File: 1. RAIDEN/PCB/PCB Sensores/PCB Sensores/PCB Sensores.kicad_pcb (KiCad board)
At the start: 2 copper layers, 61.4 x 100 mm, 19 parts, among them J2 LEDS_1, J3 LEDS_1, J4 LEDS_1, U1 BOB-09056

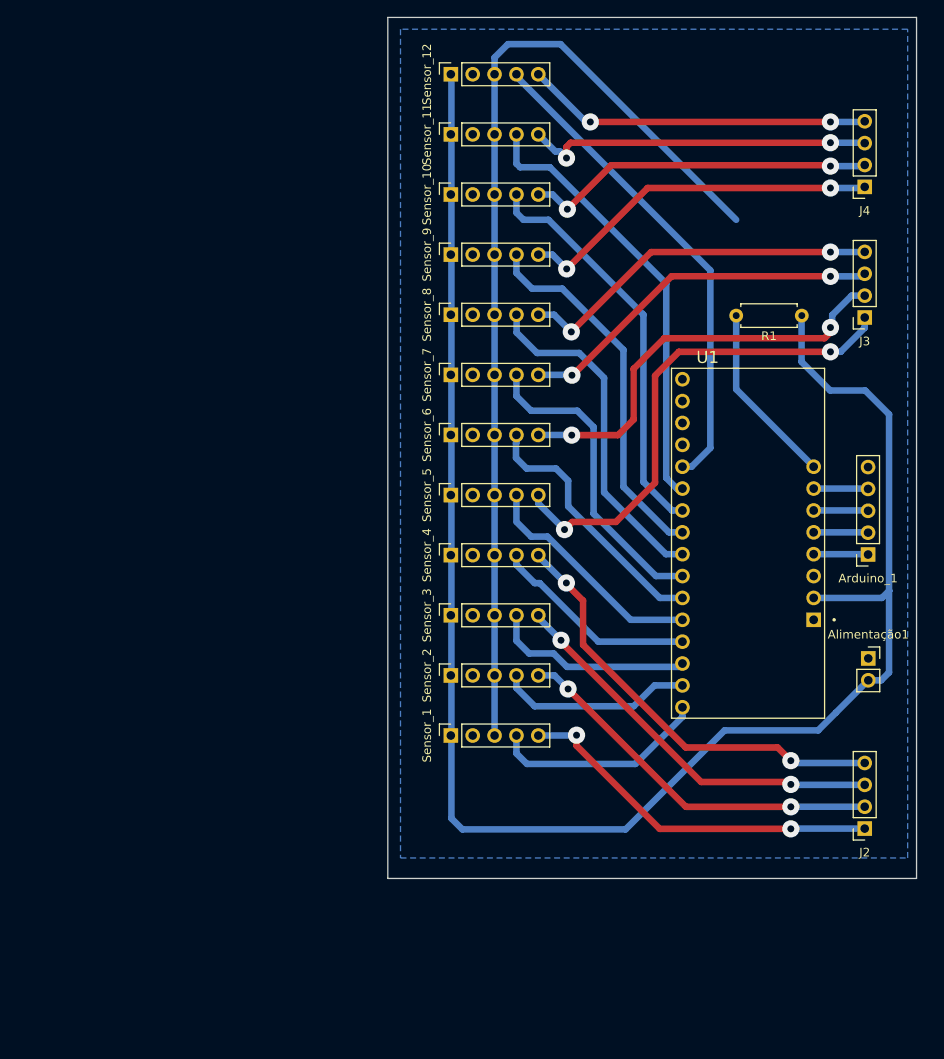
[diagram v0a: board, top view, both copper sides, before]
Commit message: V2 da PCB dos sensores
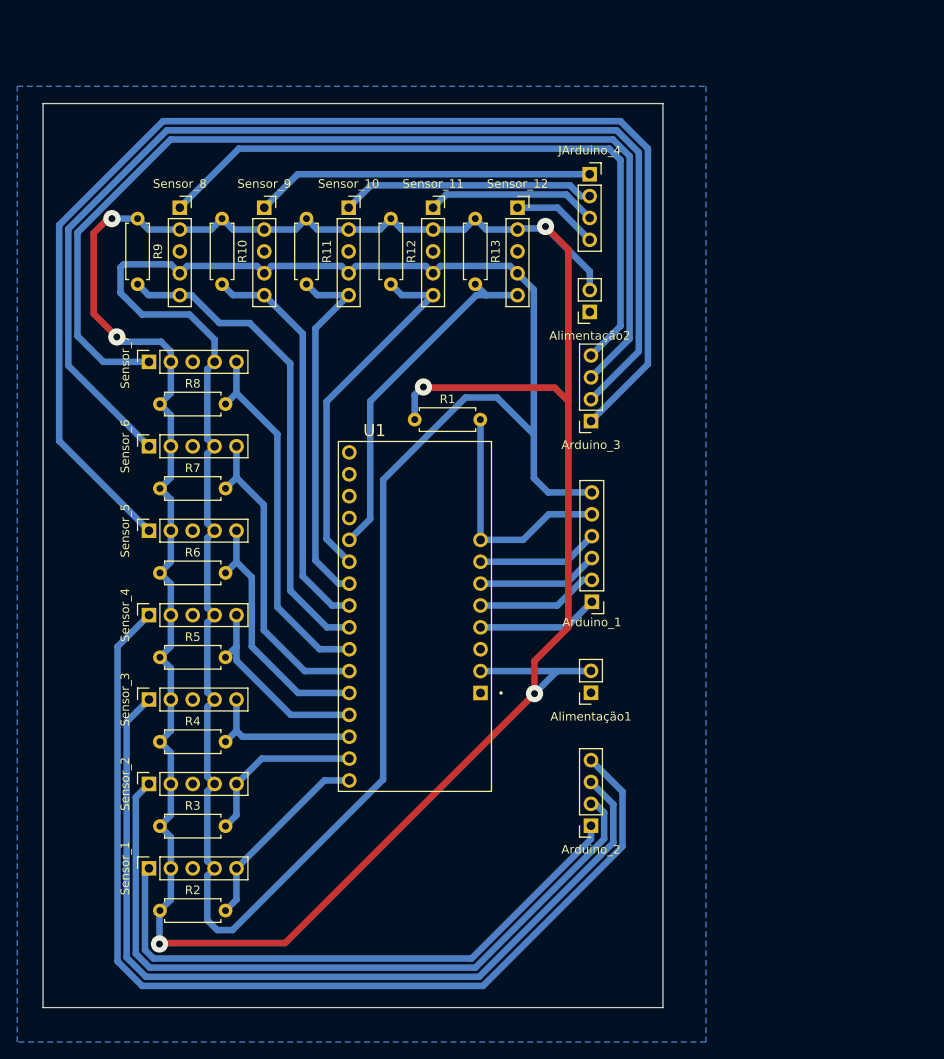
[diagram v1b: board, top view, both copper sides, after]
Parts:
- removed J2, J3, J4: LEDS_1, Connector_PinSocket_2.54mm:PinSocket_1x04_P2.54mm_Vertical
- added Alimentação2: Conn_01x02, Connector_PinSocket_2.54mm:PinSocket_1x02_P2.54mm_Vertical, F.Cu at (151.5, 64.2)
- added Arduino_2: LEDS_1, Connector_PinSocket_2.54mm:PinSocket_1x04_P2.54mm_Vertical, F.Cu at (151.6, 123.9)
- added Arduino_3: LEDS_1, Connector_PinSocket_2.54mm:PinSocket_1x04_P2.54mm_Vertical, F.Cu at (151.6, 76.9)
- added JArduino_4: LEDS_1, Connector_PinSocket_2.54mm:PinSocket_1x04_P2.54mm_Vertical, F.Cu at (151.5, 48.2)
- added R10: R, Resistor_THT:R_Axial_DIN0207_L6.3mm_D2.5mm_P7.62mm_Horizontal, F.Cu at (108.8, 53.4)
- added R11: R, Resistor_THT:R_Axial_DIN0207_L6.3mm_D2.5mm_P7.62mm_Horizontal, F.Cu at (118.6, 53.4)
- added R12: R, Resistor_THT:R_Axial_DIN0207_L6.3mm_D2.5mm_P7.62mm_Horizontal, F.Cu at (128.4, 53.4)
- added R13: R, Resistor_THT:R_Axial_DIN0207_L6.3mm_D2.5mm_P7.62mm_Horizontal, F.Cu at (138.2, 53.4)
- added R2: R, Resistor_THT:R_Axial_DIN0207_L6.3mm_D2.5mm_P7.62mm_Horizontal, F.Cu at (101.6, 133.7)
- added R3: R, Resistor_THT:R_Axial_DIN0207_L6.3mm_D2.5mm_P7.62mm_Horizontal, F.Cu at (101.6, 123.9)
- added R4: R, Resistor_THT:R_Axial_DIN0207_L6.3mm_D2.5mm_P7.62mm_Horizontal, F.Cu at (101.6, 114.1)
- added R5: R, Resistor_THT:R_Axial_DIN0207_L6.3mm_D2.5mm_P7.62mm_Horizontal, F.Cu at (101.6, 104.3)
- added R6: R, Resistor_THT:R_Axial_DIN0207_L6.3mm_D2.5mm_P7.62mm_Horizontal, F.Cu at (101.6, 94.5)
- added R7: R, Resistor_THT:R_Axial_DIN0207_L6.3mm_D2.5mm_P7.62mm_Horizontal, F.Cu at (101.6, 84.7)
- added R8: R, Resistor_THT:R_Axial_DIN0207_L6.3mm_D2.5mm_P7.62mm_Horizontal, F.Cu at (101.6, 74.9)
- added R9: R, Resistor_THT:R_Axial_DIN0207_L6.3mm_D2.5mm_P7.62mm_Horizontal, F.Cu at (99.0, 53.4)
- Arduino_1: value Conn_01x05 -> Conn_01x06; footprint Connector_PinSocket_2.54mm:PinSocket_1x05_P2.54mm_Vertical -> Connector_PinHeader_2.54mm:PinHeader_1x06_P2.54mm_Vertical
- moved R1 46.6 mm to (131.2, 76.7), turned to 0 degrees
- moved U1 39.6 mm to (131.2, 99.6)
- moved Sensor_1 38.3 mm to (100.3, 128.8)
- moved Sensor_2 37.3 mm to (100.3, 119.0)
- moved Sensor_3 36.4 mm to (100.3, 109.2)
- moved Sensor_4 35.7 mm to (100.3, 99.4)
- moved Sensor_5 35.3 mm to (100.3, 89.6)
- moved Sensor_7 35.1 mm to (100.3, 70.0)
- moved Sensor_6 35.1 mm to (100.3, 79.8)
- moved Sensor_8 33.8 mm to (103.9, 52.1), turned to 0 degrees
- moved Arduino_1 32.5 mm to (151.7, 97.9)
- moved Alimentação1 32.5 mm to (151.6, 108.4), turned to 180 degrees
- moved Sensor_9 22.3 mm to (113.7, 52.1), turned to 0 degrees
- moved Sensor_12 17.3 mm to (143.1, 52.1), turned to 0 degrees
- moved Sensor_10 12.0 mm to (123.5, 52.1), turned to 0 degrees
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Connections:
- net /*2 renamed Net-(Arduino_1-Pin_4)
- net /*3 renamed Net-(Arduino_1-Pin_3)
- net /*4 renamed Net-(Arduino_1-Pin_2)
- net /*5 renamed Net-(Arduino_1-Pin_1)
- Arduino_1 pad 5: SCL -> SDA
- Sensor_1 pad 1: VIN -> LED_1
- Sensor_1 pad 2: GND -> VIN
- Sensor_1 pad 3: SCL -> GND
- Sensor_1 pad 4: SDA_1 -> SCL
- Sensor_1 pad 5: LED_1 -> SDA_1
- Sensor_10 pad 1: VIN -> LED_10
- Sensor_10 pad 2: GND -> VIN
- Sensor_10 pad 3: SCL -> GND
- Sensor_10 pad 4: SDA_10 -> SCL
- Sensor_10 pad 5: LED_10 -> SDA_10
- Sensor_11 pad 1: VIN -> LED_11
- Sensor_11 pad 2: GND -> VIN
- Sensor_11 pad 3: SCL -> GND
- Sensor_11 pad 4: SDA_11 -> SCL
- Sensor_11 pad 5: LED_11 -> SDA_11
- Sensor_12 pad 1: VIN -> LED_12
- Sensor_12 pad 2: GND -> VIN
- Sensor_12 pad 3: SCL -> GND
- Sensor_12 pad 4: SDA_12 -> SCL
- Sensor_12 pad 5: LED_12 -> SDA_12
- Sensor_2 pad 1: VIN -> LED_2
- Sensor_2 pad 2: GND -> VIN
- Sensor_2 pad 3: SCL -> GND
- Sensor_2 pad 4: SDA_2 -> SCL
- Sensor_2 pad 5: LED_2 -> SDA_2
- Sensor_3 pad 1: VIN -> LED_3
- Sensor_3 pad 2: GND -> VIN
- Sensor_3 pad 3: SCL -> GND
- Sensor_3 pad 4: SDA_3 -> SCL
- Sensor_3 pad 5: LED_3 -> SDA_3
- Sensor_4 pad 1: VIN -> LED_4
- Sensor_4 pad 2: GND -> VIN
- Sensor_4 pad 3: SCL -> GND
- Sensor_4 pad 4: SDA_4 -> SCL
- Sensor_4 pad 5: LED_4 -> SDA_4
- Sensor_5 pad 1: VIN -> LED_5
- Sensor_5 pad 2: GND -> VIN
- Sensor_5 pad 3: SCL -> GND
- Sensor_5 pad 4: SDA_5 -> SCL
- Sensor_5 pad 5: LED_5 -> SDA_5
- Sensor_6 pad 1: VIN -> LED_6
- Sensor_6 pad 2: GND -> VIN
- Sensor_6 pad 3: SCL -> GND
- Sensor_6 pad 4: SDA_6 -> SCL
- Sensor_6 pad 5: LED_6 -> SDA_6
- Sensor_7 pad 1: VIN -> LED_7
- Sensor_7 pad 2: GND -> VIN
- Sensor_7 pad 3: SCL -> GND
- Sensor_7 pad 4: SDA_7 -> SCL
- Sensor_7 pad 5: LED_7 -> SDA_7
- Sensor_8 pad 1: VIN -> LED_8
- Sensor_8 pad 2: GND -> VIN
- Sensor_8 pad 3: SCL -> GND
- Sensor_8 pad 4: SDA_8 -> SCL
- Sensor_8 pad 5: LED_8 -> SDA_8
- Sensor_9 pad 1: VIN -> LED_9
- Sensor_9 pad 2: GND -> VIN
- Sensor_9 pad 3: SCL -> GND
- Sensor_9 pad 4: SDA_9 -> SCL
- Sensor_9 pad 5: LED_9 -> SDA_9
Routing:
- net SCL: track 116.0 -> 255.8 mm
- net VIN: track 202.5 -> 314.2 mm, vias 0 -> 6
- net LED_5: track 58.3 -> 148.9 mm, vias 2 -> 0
- net LED_6: track 49.3 -> 132.2 mm, vias 2 -> 0
- net LED_7: track 42.6 -> 118.5 mm, vias 2 -> 0
- net LED_4: track 51.0 -> 119.8 mm, vias 2 -> 0
- net LED_3: track 46.3 -> 103.1 mm, vias 2 -> 0
- net LED_2: track 44.4 -> 86.6 mm, vias 2 -> 0
- net LED_8: track 42.6 -> 78.7 mm, vias 2 -> 0
- net LED_12: track 40.2 -> 9.93 mm, vias 2 -> 0
- net LED_1: track 43.4 -> 69.2 mm, vias 2 -> 0
- net LED_11: track 40.6 -> 19.9 mm, vias 2 -> 0
- net SDA_8: track 39.6 -> 56.5 mm
- net SDA_12: track 56.9 -> 41.1 mm
- net LED_10: track 41.3 -> 29.6 mm, vias 2 -> 0
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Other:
- board size 61.4 x 100 mm -> 72 x 105 mm
